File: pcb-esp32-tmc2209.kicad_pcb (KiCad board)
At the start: 2 copper layers, 75.5 x 71 mm, 16 parts, among them J1 Conn_01x04_Pin, J2 12V Terminal, J3 5V Terminal, J4 Extra Pins, J5 Button 1, J6 Button 2, J7 PINHD_1x12_Male, J8 12V Output, U1 nanoESP32-C6

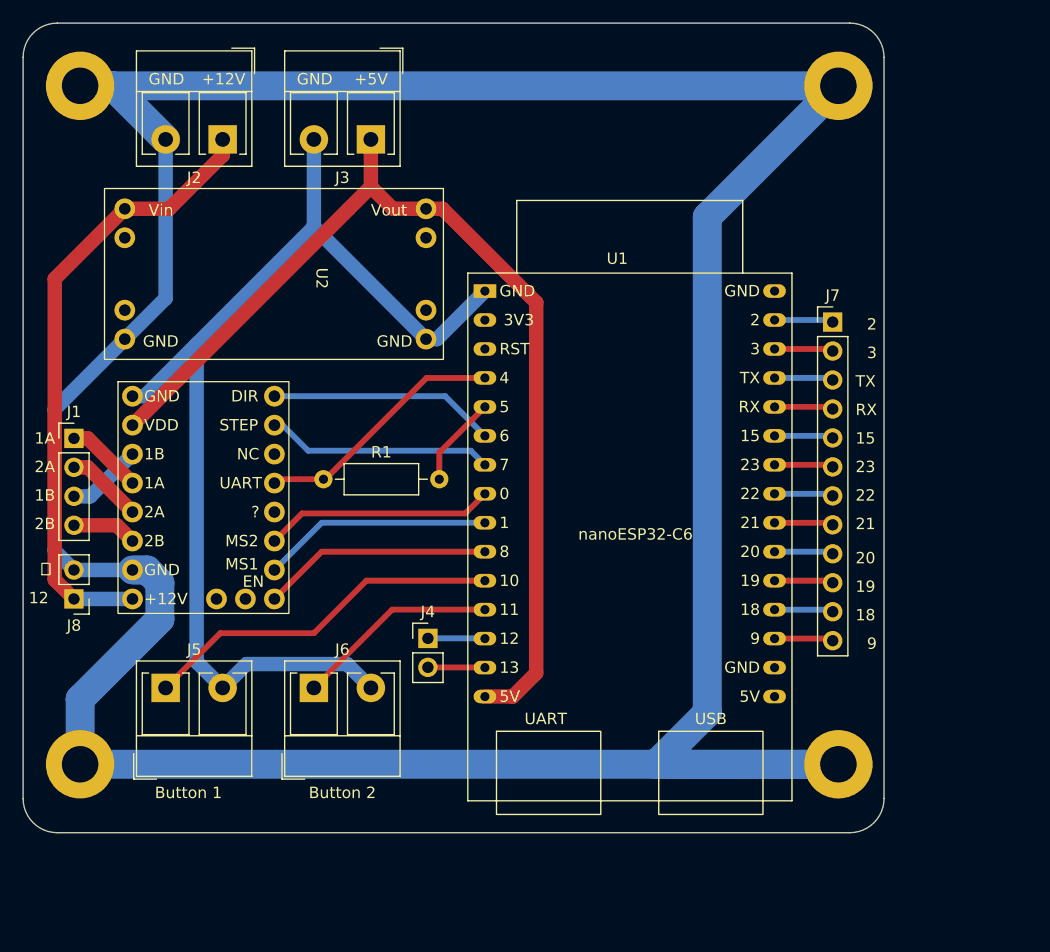
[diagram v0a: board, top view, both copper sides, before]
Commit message: initial commit of version 2
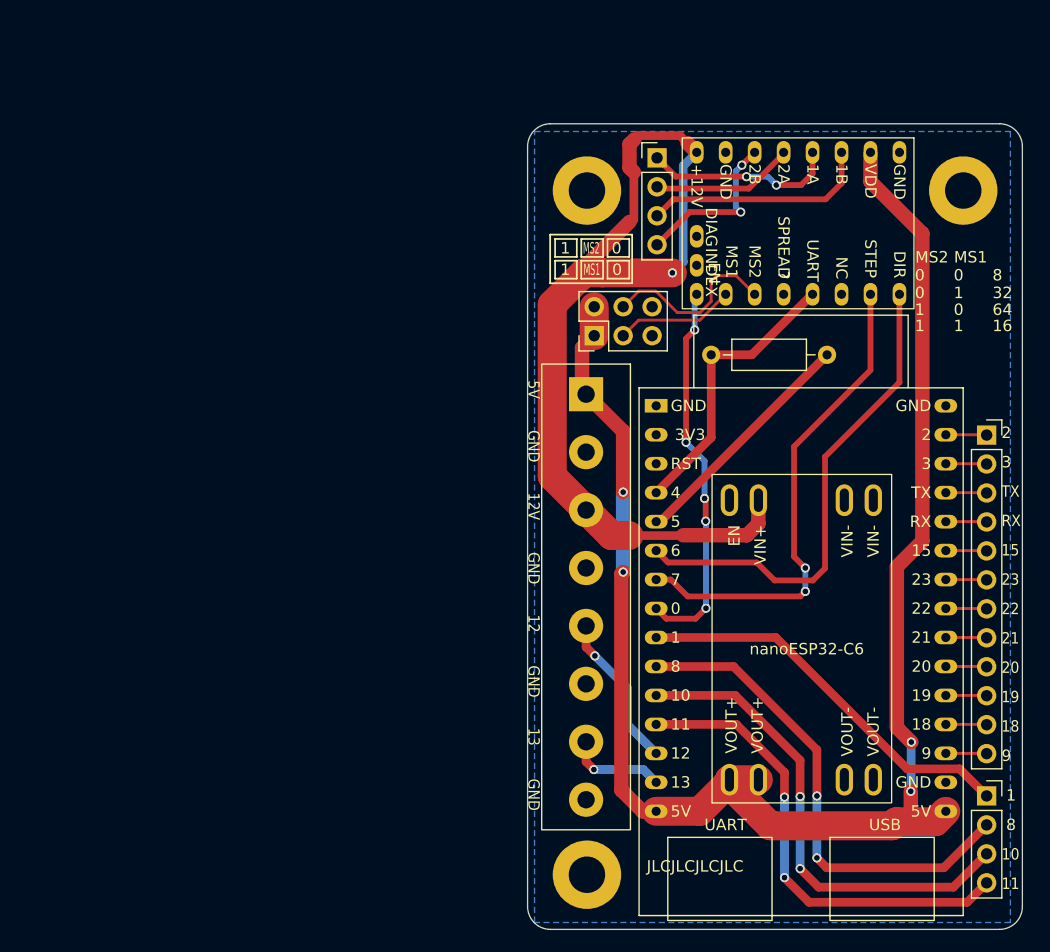
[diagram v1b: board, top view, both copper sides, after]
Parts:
- removed H4: MountingHole_M3, PCM_SL_Mechanical:MountingHole_3.2mm_Pad
- removed J4: Extra Pins, Connector_PinHeader_2.54mm:PinHeader_1x02_P2.54mm_Vertical
- removed J7: PINHD_1x12_Male, Connector_PinHeader_2.54mm:PinHeader_1x12_P2.54mm_Vertical
- removed J8: 12V Output, Connector_PinHeader_2.54mm:PinHeader_1x02_P2.54mm_Vertical
- added G***: LOGO, LOGO, B.Cu at (139.7, 105.1)
- J2: value 12V Terminal -> Screw_Terminal_8_P5.00mm; footprint TerminalBlock_RND:TerminalBlock_RND_205-00276_1x02_P5.00mm_Vertical -> TerminalBlock:TerminalBlock_bornier-8_P5.08mm
- J3: value 5V Terminal -> PINHD_1x12_Female; footprint TerminalBlock_RND:TerminalBlock_RND_205-00276_1x02_P5.00mm_Vertical -> Connector_PinSocket_2.54mm:PinSocket_1x12_P2.54mm_Vertical
- J5: value Button 1 -> Microstep Selector; footprint TerminalBlock_RND:TerminalBlock_RND_205-00276_1x02_P5.00mm_Vertical -> Connector_PinHeader_2.54mm:PinHeader_2x03_P2.54mm_Vertical
- J6: value Button 2 -> PINHD_1x4_Female; footprint TerminalBlock_RND:TerminalBlock_RND_205-00276_1x02_P5.00mm_Vertical -> Connector_PinSocket_2.54mm:PinSocket_1x04_P2.54mm_Vertical
- U2: footprint CustomComponents:BuckConverter -> CustomComponents:V100-EY9 DC-DC Converter
- moved H3 82.2 mm to (118.9, 129.2)
- moved TMC2209 66.3 mm to (138.7, 65.8), turned to -90 degrees
- moved J3 59.9 mm to (154.0, 90.6), turned to 0 degrees
- moved J6 59.8 mm to (154.0, 122.3)
- moved U2 57.1 mm to (131.4, 121.4), turned to 90 degrees
- moved J1 56.7 mm to (125.1, 66.3)
- moved H2 51.5 mm to (151.9, 69.2)
- moved J5 48.6 mm to (119.6, 81.9), turned to 90 degrees
- moved J2 38.9 mm to (118.9, 87.0), turned to -90 degrees
- moved R1 35.7 mm to (129.8, 83.6)
- moved H1 23.9 mm to (118.9, 69.2)
- moved U1 18.1 mm to (125.0, 88.1)
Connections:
- J2 pad 1: +12V -> +5V
- J3 pad 1: Net-(J3-Pin_1) -> Net-(U1-2)
- J3 pad 2: Net-(J3-Pin_2) -> Net-(U1-3)
- J5 pad 1: Net-(J5-Pin_1) -> +5V
- J5 pad 2: Net-(J3-Pin_2) -> +5V
- J6 pad 1: Net-(J6-Pin_1) -> Net-(U1-1)
- J6 pad 2: Net-(J3-Pin_2) -> Net-(U1-8)
- TMC2209 pad 1: Net-(J3-Pin_2) -> GND
- TMC2209 pad 2: Net-(J3-Pin_1) -> +5V
- U1 pad 1: Net-(J3-Pin_2) -> GND
- U1 pad 10: Net-(TMC2209-EN) -> Net-(U1-8)
- U1 pad 11: Net-(J5-Pin_1) -> Net-(U1-10)
- U1 pad 12: Net-(J6-Pin_1) -> Net-(U1-11)
- U1 pad 15: Net-(J3-Pin_1) -> +5V
- U1 pad 16: unconnected-(U1-GND-Pad16) -> GND
- U1 pad 29: unconnected-(U1-GND-Pad29) -> GND
- U1 pad 30: unconnected-(U1-5V-Pad30) -> +5V
- U1 pad 8: Net-(TMC2209-MS2) -> Net-(TMC2209-EN)
- U1 pad 9: Net-(TMC2209-MS1) -> Net-(U1-1)
- U2 pad 1: +12V -> +5V
- U2 pad 3: Net-(J3-Pin_1) -> unconnected-(U2-EN-Pad3)
- U2 pad 4: Net-(J3-Pin_2) -> +12V
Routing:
- net GND: track 293.9 -> 0.00 mm
- net +5V: track 0.00 -> 143.0 mm, vias 0 -> 4
- net Net-(J3-Pin_2): track 96.5 -> 0.00 mm
- net Net-(J3-Pin_1): track 90.3 -> 0.00 mm
- net Net-(U1-8): track 0.00 -> 43.4 mm, vias 0 -> 2
- net Net-(U1-10): track 0.00 -> 42.7 mm, vias 0 -> 2
- net Net-(U1-11): track 0.00 -> 41.5 mm, vias 0 -> 2
- net Net-(U1-1): track 0.00 -> 34.7 mm
- net Net-(J5-Pin_1): track 31.9 -> 0.00 mm
- net +12V: track 54.5 -> 80.7 mm, vias 0 -> 1
- net Net-(TMC2209-STEP): track 19.9 -> 43.1 mm, vias 0 -> 2
- net Net-(TMC2209-DIR): track 19.9 -> 43.1 mm
- net Net-(J6-Pin_1): track 17.8 -> 0.00 mm
- net Net-(TMC2209-EN): track 20.2 -> 33.8 mm, vias 0 -> 5
- net Net-(J1-Pin_3): track 6.67 -> 20.1 mm
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- added copper zone on B.Cu, net GND
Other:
- board size 75.5 x 71 mm -> 43.4 x 70.7 mm
- board text added: "0"
- board text added: "1"
- board text added: "10"
- board text added: "11"
- board text added: "12V"
- board text added: "13"
- board text added: "16"
- board text added: "32"
- board text added: "5V"
- board text added: "6"
- board text added: "64"
- board text added: "8"
- board text added: "JLCJLCJLCJLC"
- board text added: "MS1"
- board text added: "MS2"
- board text removed: "+12V"
- board text removed: "+5V"
- board text removed: "1A"
- board text removed: "1B"
- board text removed: "2A"
- board text removed: "2B"
- board text removed: "Vin"
- board text removed: "Vout"
- board text removed: "⏚"
